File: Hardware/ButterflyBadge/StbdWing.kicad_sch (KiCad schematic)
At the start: 266 parts, among them J1 Conn_01x06, J4 Conn_01x08, U1 XC6206PxxxMR, U5 SN74LV1T34DBV

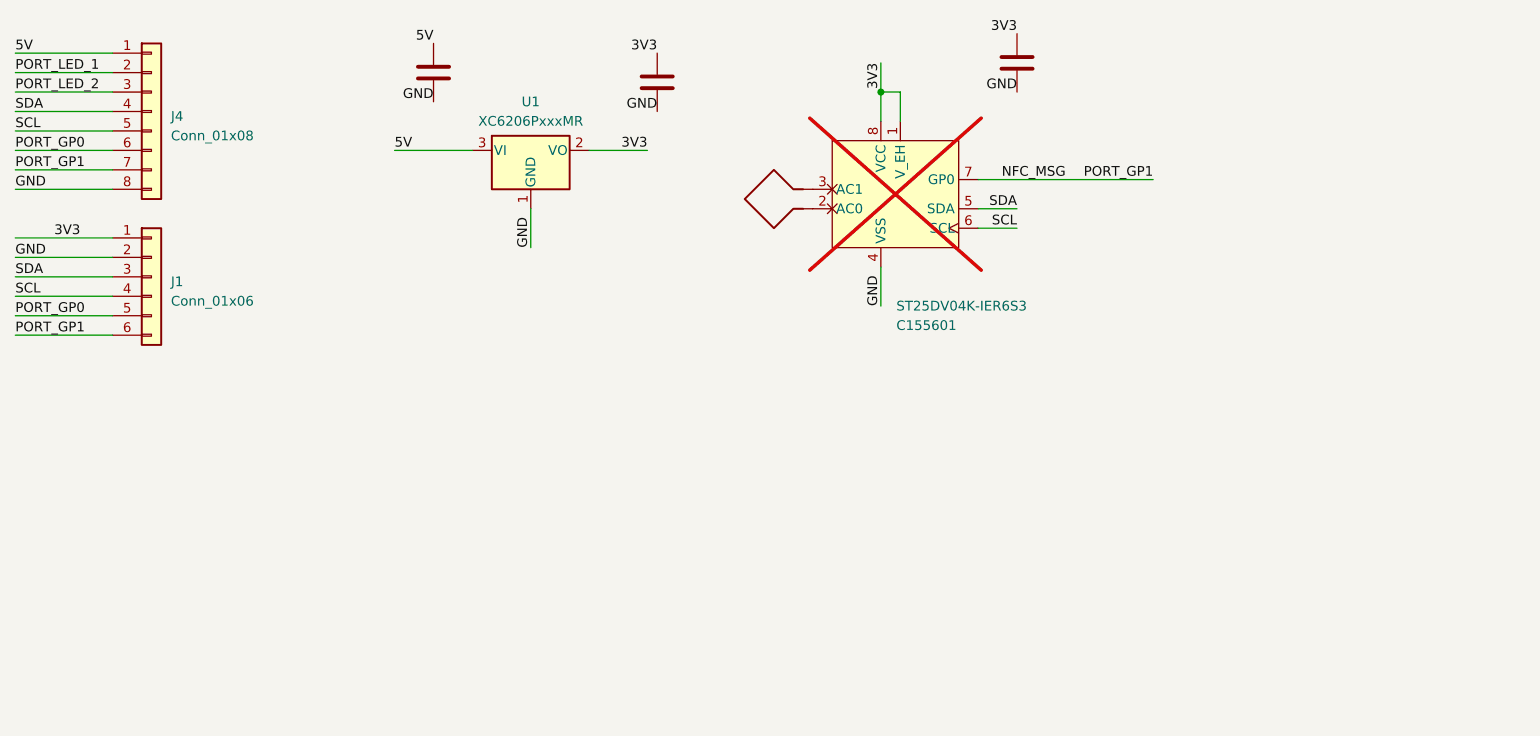
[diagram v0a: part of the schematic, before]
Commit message: Schematic is done! Now to work on the main PCB
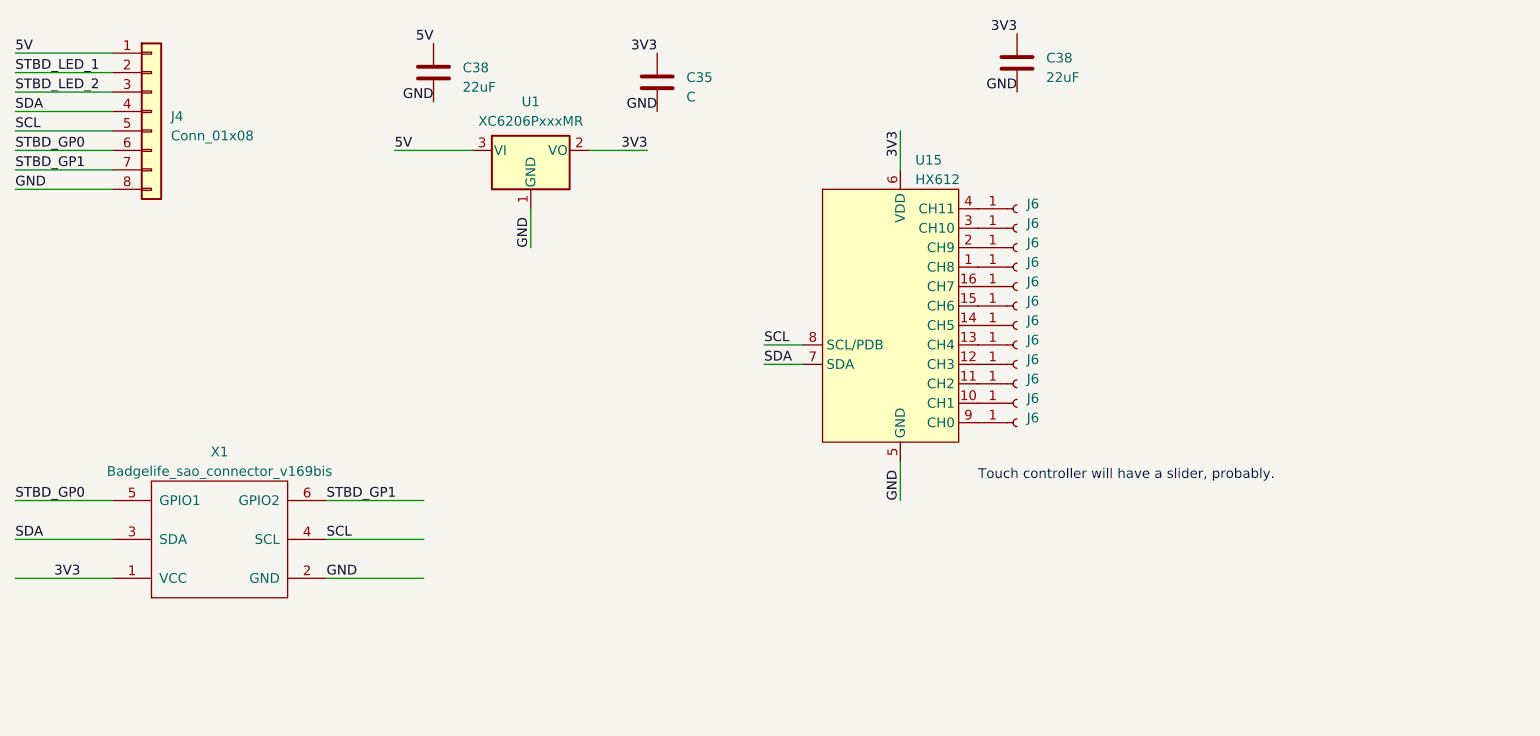
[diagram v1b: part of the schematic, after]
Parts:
- removed ? (x3): (no value), symbol Device:C
- removed ?: (no value), symbol Device:Antenna_Loop
- removed ?: (no value), symbol ST25DV04K:ST25DV04K
- removed J1: Conn_01x06, symbol Connector_Generic:Conn_01x06
- added C35: C, symbol Device:C
- added C38 (x2): 22uF, symbol Device:C
- added J6 (x12): Conn_01x01_Female, symbol Connector:Conn_01x01_Female
- added U15: HX612, Package_SO:SOP-16_3.9x9.9mm_P1.27mm, symbol HX612:HX612
- added X1: Badgelife_sao_connector_v169bis, badgelife_sao_v169bis:Badgelife-SAOv169-BADGE-2x3, symbol badgelife_shitty_addon_v169bis:Badgelife_sao_connector_v169bis
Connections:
- net 3V3: now also C35.1, C38.1, U15.6 (VDD), X1.1 (VCC)
- net 5V: now also C38.1
- net GND: now also C35.2, C38.2, C38.2, U15.5 (GND), X1.2 (GND)
- net PORT_LED_1: no longer J4.2 (Pin_2)
- net PORT_LED_2: no longer J4.3 (Pin_3)
- net SCL: now also U15.8 (SCL/PDB), X1.4 (SCL)
- net SDA: now also U15.7 (SDA), X1.3 (SDA)
- net NFC_MSG renamed STBD_GP1
- net STBD_GP1: now also X1.6 (GPIO2)
- net PORT_GP0 renamed STBD_GP0
- net STBD_GP0: now also X1.5 (GPIO1)
- new net: J6.1 (Pin_1), U15.1 (CH8)
- new net: J6.1 (Pin_1), U15.10 (CH1)
- new net: J6.1 (Pin_1), U15.11 (CH2)
- new net: J6.1 (Pin_1), U15.12 (CH3)
- new net: J6.1 (Pin_1), U15.13 (CH4)
- new net: J6.1 (Pin_1), U15.14 (CH5)
- new net: J6.1 (Pin_1), U15.15 (CH6)
- new net: J6.1 (Pin_1), U15.16 (CH7)
- new net: J6.1 (Pin_1), U15.2 (CH9)
- new net: J6.1 (Pin_1), U15.3 (CH10)
- new net: J6.1 (Pin_1), U15.4 (CH11)
- new net: J6.1 (Pin_1), U15.9 (CH0)
- new net STBD_LED_1: J4.2 (Pin_2)
- new net STBD_LED_2: J4.3 (Pin_3)
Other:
- note added: "Touch controller will have a slider, probably."

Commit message: Hardware mods
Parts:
- D2: Manufacturer PN C2890364 -> (none)
